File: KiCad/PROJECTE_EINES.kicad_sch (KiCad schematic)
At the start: 5 parts

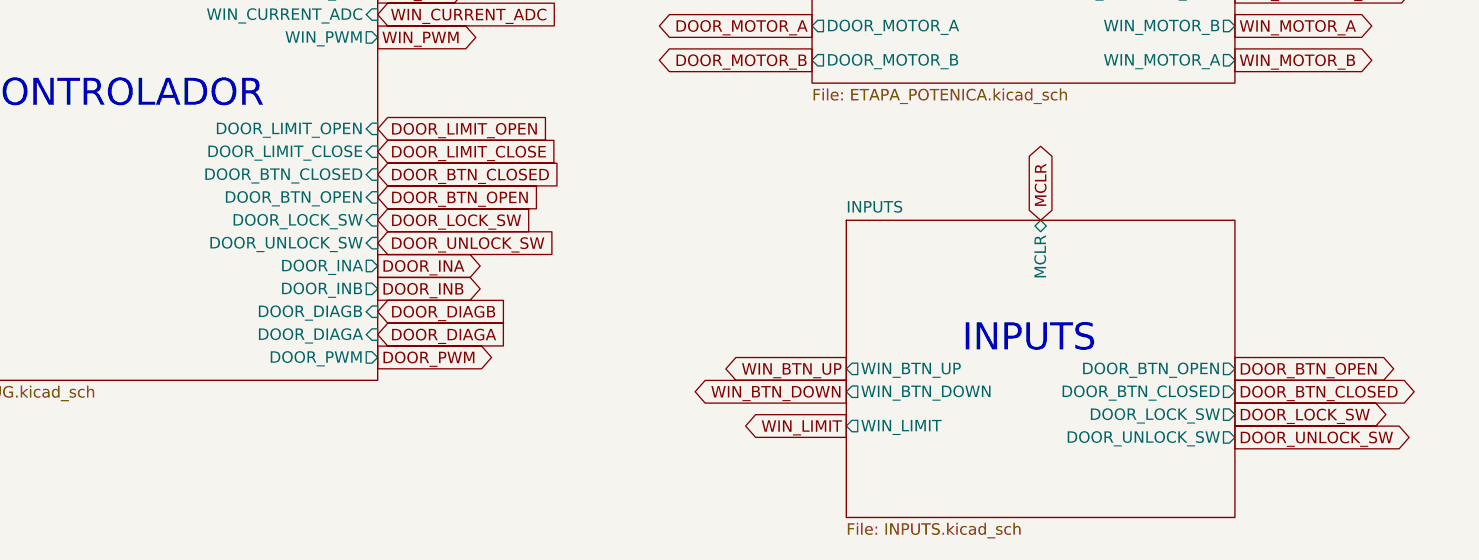
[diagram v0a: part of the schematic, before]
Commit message: Inputs
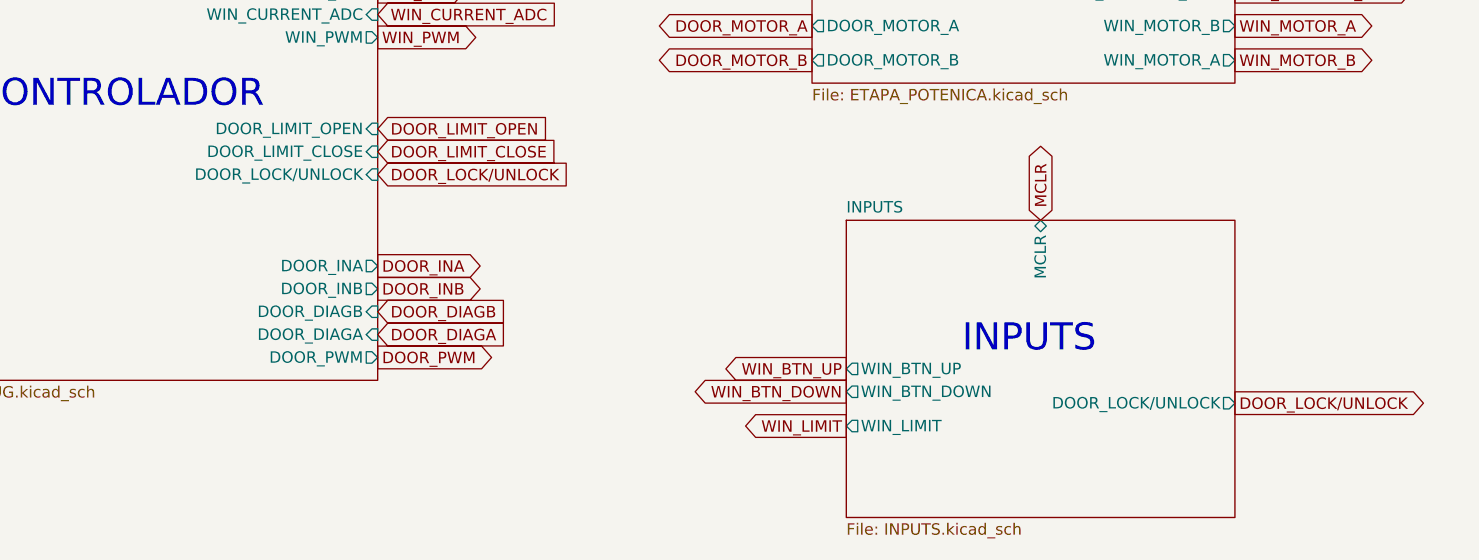
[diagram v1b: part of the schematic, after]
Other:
- sheet INPUTS ports: added DOOR_LOCK/UNLOCK; removed DOOR_BTN_CLOSED, DOOR_BTN_OPEN, DOOR_LOCK_SW, DOOR_UNLOCK_SW
- sheet MICROCONTROLADOR I DEBUG ports: added DOOR_LOCK/UNLOCK; removed DOOR_BTN_CLOSED, DOOR_BTN_OPEN, DOOR_LOCK_SW, DOOR_UNLOCK_SW
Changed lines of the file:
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@@
-		)
-	)
-	(global_label "DOOR_LOCK_SW"
-		(shape input)
-		(at 153.67 125.73 0)
-		(effects
-			(font
-				(size 1.27 1.27)
-			)
-			(justify left)
-		)
-		(property "Intersheetrefs" "${INTERSHEET_REFS}"
-			(at 153.67 125.73 0)
-			(effects
-				(font
-					(size 1.27 1.27)
-				)
-				(hide yes)
-			)
-		)
-	)
-	(global_label "DOOR_LOCK_SW"
-		(shape output)
-		(at 248.92 147.32 0)
-		(effects
-			(font
-				(size 1.27 1.27)
-			)
-			(justify left)
-		)
-		(property "Intersheetrefs" "${INTERSHEET_REFS}"
-			(at 248.92 147.32 0)
-			(effects
-				(font
-					(size 1.27 1.27)
-				)
-				(hide yes)
-			)
 		)
 	)
@@
 		(property "Intersheetrefs" "${INTERSHEET_REFS}"
 			(at 248.92 76.2 0)
-			(effects
-				(font
-					(size 1.27 1.27)
-				)
-				(hide yes)
-			)
-		)
-	)
-	(global_label "DOOR_BTN_OPEN"
-		(shape input)
-		(at 153.67 123.19 0)
-		(effects
-			(font
-				(size 1.27 1.27)
-			)
-			(justify left)
-		)
-		(property "Intersheetrefs" "${INTERSHEET_REFS}"
-			(at 153.67 123.19 0)
 			(effects
 				(font
@@
 		)
 	)
-	(global_label "DOOR_UNLOCK_SW"
-		(shape output)
-		(at 248.92 149.86 0)
-		(effects
-			(font
-				(size 1.27 1.27)
-			)
-			(justify left)
-		)
-		(property "Intersheetrefs" "${INTERSHEET_REFS}"
-			(at 248.92 149.86 0)
-			(effects
-				(font
-					(size 1.27 1.27)
-				)
-				(hide yes)
-			)
-		)
-	)
 	(global_label "UART_TX"
 		(shape output)
@@
 		(property "Intersheetrefs" "${INTERSHEET_REFS}"
 			(at 82.55 113.03 0)
-			(effects
-				(font
-					(size 1.27 1.27)
-				)
-				(hide yes)
-			)
-		)
-	)
-	(global_label "DOOR_UNLOCK_SW"
-		(shape input)
-		(at 153.67 128.27 0)
-		(effects
-			(font
-				(size 1.27 1.27)
-			)
-			(justify left)
-		)
-		(property "Intersheetrefs" "${INTERSHEET_REFS}"
-			(at 153.67 128.27 0)
 			(effects
 				(font
@@
 		)
 	)
-	(global_label "DOOR_BTN_CLOSED"
-		(shape input)
-		(at 153.67 120.65 0)
-		(effects
-			(font
-				(size 1.27 1.27)
-			)
-			(justify left)
-		)
-		(property "Intersheetrefs" "${INTERSHEET_REFS}"
-			(at 153.67 120.65 0)
-			(effects
-				(font
-					(size 1.27 1.27)
-				)
-				(hide yes)
-			)
-		)
-	)
 	(global_label "WIN_MOTOR_A"
 		(shape output)
@@
 		)
 	)
-	(global_label "DOOR_BTN_CLOSED"
-		(shape output)
-		(at 248.92 144.78 0)
-		(effects
-			(font
-				(size 1.27 1.27)
-			)
-			(justify left)
-		)
-		(property "Intersheetrefs" "${INTERSHEET_REFS}"
-			(at 248.92 144.78 0)
-			(effects
-				(font
-					(size 1.27 1.27)
-				)
-				(hide yes)
-			)
-		)
-	)
 	(global_label "DOOR_MOTOR_B"
 		(shape output)
@@
 		)
 	)
-	(global_label "DOOR_BTN_OPEN"
-		(shape output)
-		(at 248.92 142.24 0)
-		(effects
-			(font
-				(size 1.27 1.27)
-			)
-			(justify left)
-		)
-		(property "Intersheetrefs" "${INTERSHEET_REFS}"
-			(at 248.92 142.24 0)
-			(effects
-				(font
-					(size 1.27 1.27)
-				)
-				(hide yes)
-			)
-		)
-	)
 	(global_label "RFID_MISO"
 		(shape input)
@@
 		)
 	)
+	(global_label "DOOR_LOCK{slash}UNLOCK"
+		(shape input)
+		(at 153.67 120.65 0)
+		(fields_autoplaced yes)
+		(effects
+			(font
+				(size 1.27 1.27)
+			)
+			(justify left)
+		)
+		(property "Intersheetrefs" "${INTERSHEET_REFS}"
+			(at 176.6125 120.65 0)
+			(effects
+				(font
+					(size 1.27 1.27)
+				)
+				(justify left)
+				(hide yes)
+			)
+		)
+	)
 	(global_label "WIN_BTN_UP"
 		(shape output)
@@
 					(size 1.27 1.27)
 				)
+				(hide yes)
+			)
+		)
+	)
+	(global_label "DOOR_LOCK{slash}UNLOCK"
+		(shape output)
+		(at 248.92 146.05 0)
+		(fields_autoplaced yes)
+		(effects
+			(font
+				(size 1.27 1.27)
+			)
+			(justify left)
+		)
+		(property "Intersheetrefs" "${INTERSHEET_REFS}"
+			(at 271.8625 146.05 0)
+			(effects
+				(font
+					(size 1.27 1.27)
+				)
+				(justify left)
 				(hide yes)
 			)
@@
 			)
 		)
-		(pin "DOOR_BTN_CLOSED" input
-			(at 153.67 120.65 0)
-			(effects
-				(font
-					(size 1.27 1.27)
-				)
-				(justify right)
-			)
-		)
-		(pin "DOOR_BTN_OPEN" input
-			(at 153.67 123.19 0)
-			(effects
-				(font
-					(size 1.27 1.27)
-				)
-				(justify right)
-			)
-		)
 		(pin "DOOR_DIAGA" input
 			(at 153.67 138.43 0)
@@
 			)
 		)
-		(pin "DOOR_LOCK_SW" input
-			(at 153.67 125.73 0)
-			(effects
-				(font
-					(size 1.27 1.27)
-				)
-				(justify right)
-			)
-		)
 		(pin "DOOR_PWM" output
 			(at 153.67 140.97 0)
@@
 			)
 		)
-		(pin "DOOR_UNLOCK_SW" input
-			(at 153.67 128.27 0)
+		(pin "DOOR_LOCK{slash}UNLOCK" input
+			(at 153.67 120.65 0)
 			(effects
 				(font
@@
 			)
 		)
-		(pin "DOOR_BTN_CLOSED" output
-			(at 248.92 144.78 0)
-			(effects
-				(font
-					(size 1.27 1.27)
-				)
-				(justify right)
-			)
-		)
-		(pin "DOOR_BTN_OPEN" output
-			(at 248.92 142.24 0)
-			(effects
-				(font
-					(size 1.27 1.27)
-				)
-				(justify right)
-			)
-		)
-		(pin "DOOR_LOCK_SW" output
-			(at 248.92 147.32 0)
-			(effects
-				(font
-					(size 1.27 1.27)
-				)
-				(justify right)
-			)
-		)
-		(pin "DOOR_UNLOCK_SW" output
-			(at 248.92 149.86 0)
-			(effects
-				(font
+		(pin "DOOR_LOCK{slash}UNLOCK" output
+			(at 248.92 146.05 0)
+			(effects
+				(font
